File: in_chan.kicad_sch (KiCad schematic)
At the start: 7 parts, among them U7 MAX31910AUI+

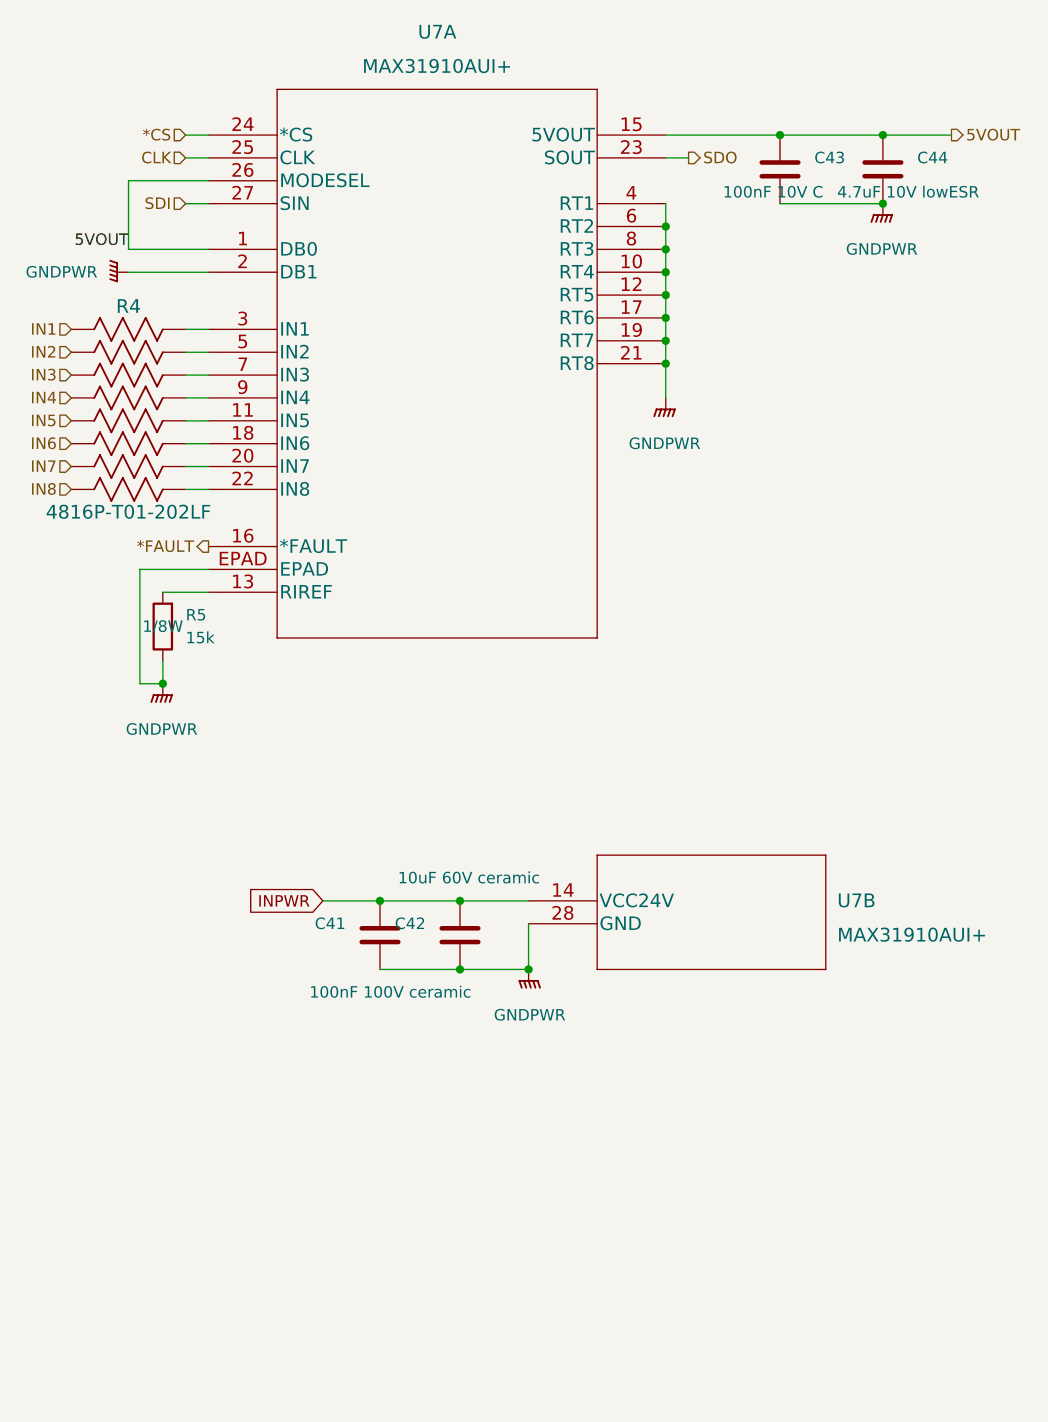
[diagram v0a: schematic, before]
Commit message: fix warnings
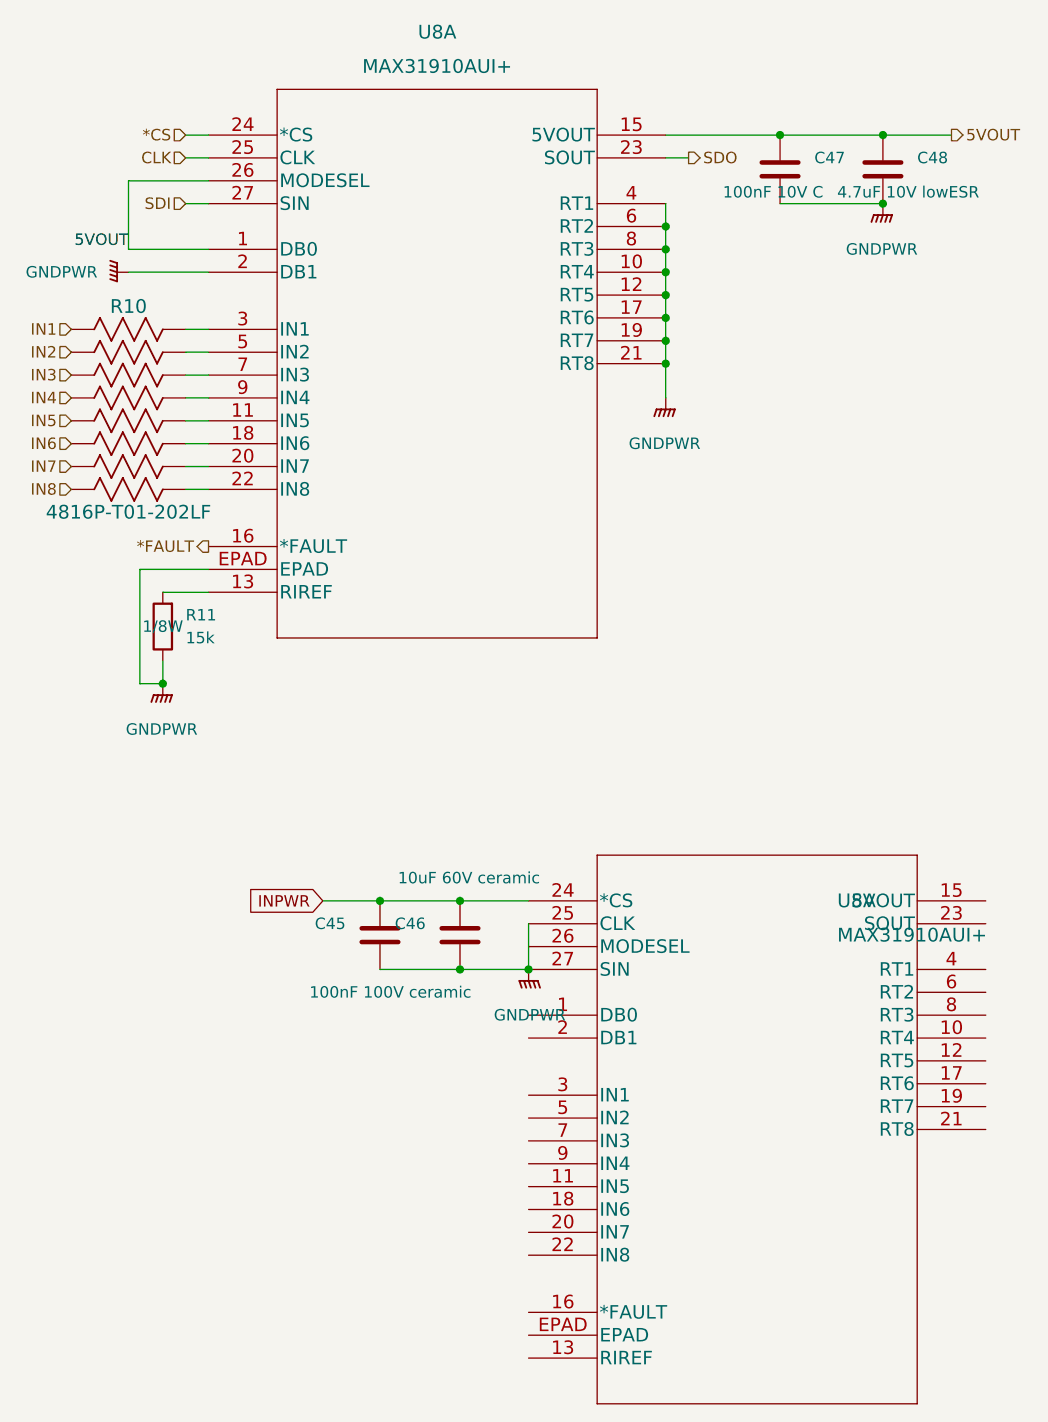
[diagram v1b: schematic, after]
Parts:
- renumbered C41 to C45, C42 to C46, C43 to C47, C44 to C48, R4 to R10, R5 to R11, U7 to U8
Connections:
- net GNDPWR: now also U8.25 (CLK), U8.27 (SIN); no longer U8.28 (GND)
- net INPWR: now also U8.24 (*CS); no longer U8.14 (VCC24V)
